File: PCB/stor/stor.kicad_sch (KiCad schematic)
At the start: 26 parts, among them J1 Conn_01x04_Socket, SW1 TS1603-TZ38HBM, SW2 TS1603-TZ38HBM, U1 STM32H723VGT6, U2 TYPE-C 24P-GTJB 040, U3 USB3300-EZK-TR, U4 TPS62177DQCR, X1 25mhz, X2 32.768k

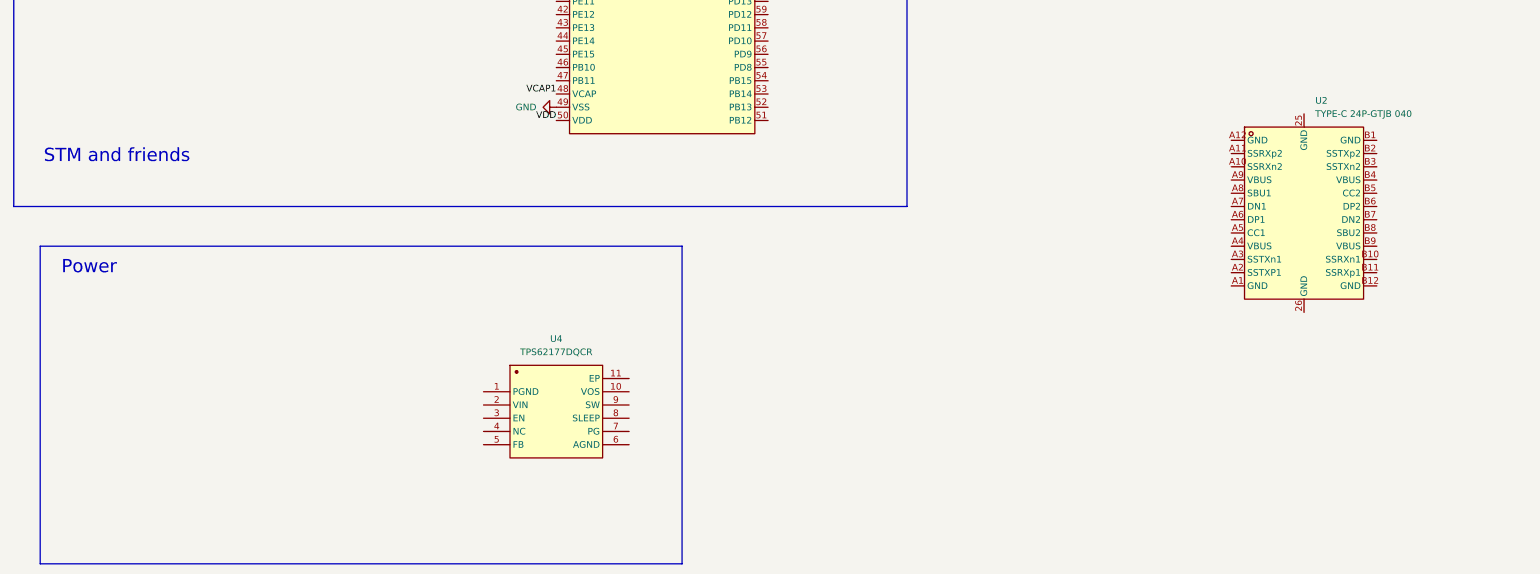
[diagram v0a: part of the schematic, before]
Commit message: pmic done
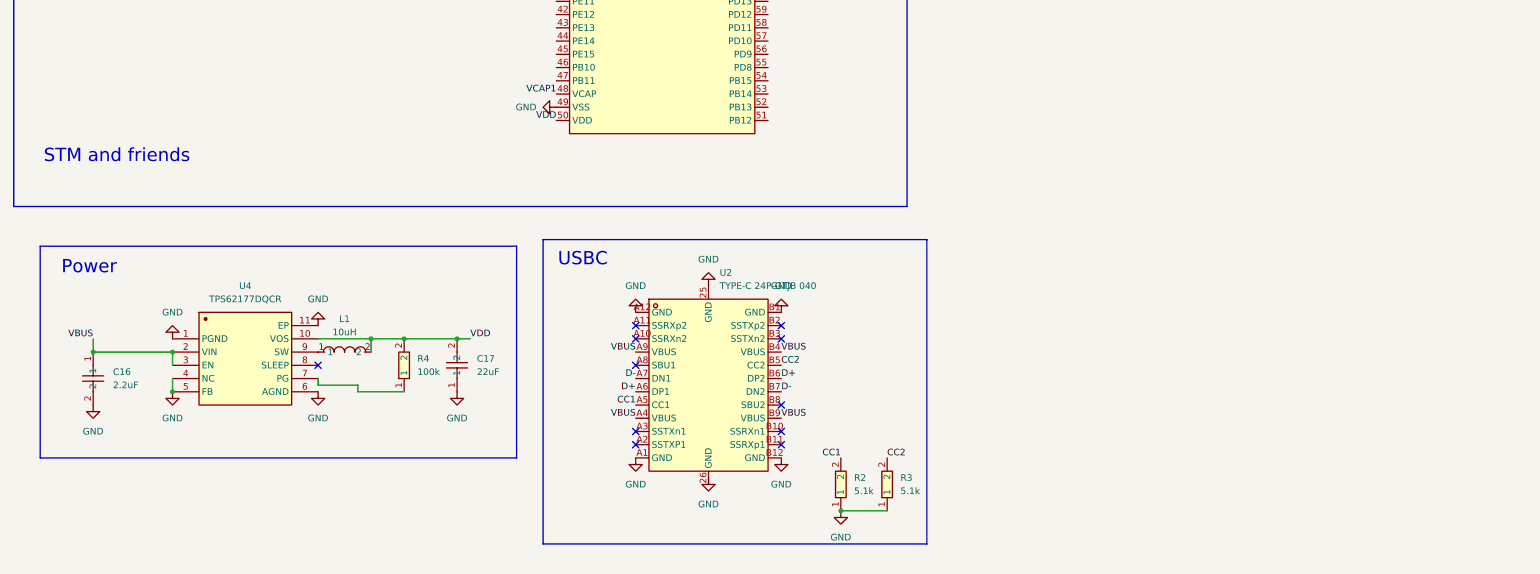
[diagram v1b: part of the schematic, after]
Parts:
- added C16: 2.2uF, easyeda2kicad:C0402, symbol easyeda2kicad:CL05A225KO5NQNC
- added C17: 22uF, easyeda2kicad:C0402, symbol easyeda2kicad:GRM158C80G226ME01D
- added L1: 10uH, easyeda2kicad:IND-SMD_L3.2-W2.5_CKST322512-2.2UH, symbol easyeda2kicad:XRTC322512S100MBCA
- added R2, R3: 5.1k, easyeda2kicad:R0402, symbol easyeda2kicad:RC0402FR-075K1L
- added R4: 100k, easyeda2kicad:R0402, symbol easyeda2kicad:RC0402FR-07100KL
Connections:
- net GND: now also U2.25 (GND), U2.A1 (GND), U2.A12 (GND), U2.B1 (GND), U2.B12 (GND), U4.1 (PGND), U4.11 (EP), U4.4 (NC), U4.5 (FB), U4.6 (AGND), C16.2, C17.1, R2.1, R3.1
- net VDD: now also U4.10 (VOS), C17.2, L1.2, R4.2
- net VBUS: now reaches U4.2 (VIN)
- net VBUS: now also U2.A4 (VBUS), U2.A9 (VBUS), U2.B4 (VBUS), U2.B9 (VBUS), U4.3 (EN), C16.1
- net at U4.7 (PG): now also R4.1
- net at U4.9 (SW): now also L1.1
- net CC1: now reaches U2.A5 (CC1)
- net CC1: now also R2.2
- net D+: now reaches U2.A6 (DP1)
- net D+: now also U2.B6 (DP2)
- net D-: now reaches U2.A7 (DN1)
- net D-: now also U2.B7 (DN2)
- net CC2: now reaches U2.B5 (CC2)
- net CC2: now also R3.2
- no-connect marks 0 -> 11
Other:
- note added: "USBC"
- moved on the sheet: U2, U4
